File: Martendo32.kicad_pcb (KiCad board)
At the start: 2 copper layers, 75.2 x 98.5 mm, 104 parts, among them CN2 ZX-MX1.25-2PWT, J1 AudioJack4_SwitchTR1, J2 Conn_01x03, J4 USB-C, Q1 NPN, Q2 AO3401A, SW1 SK-3296S-01-L3, U3 TP4056, U4 NS4168, U5 TPS61040DBV, U6 AP2112K-3.3

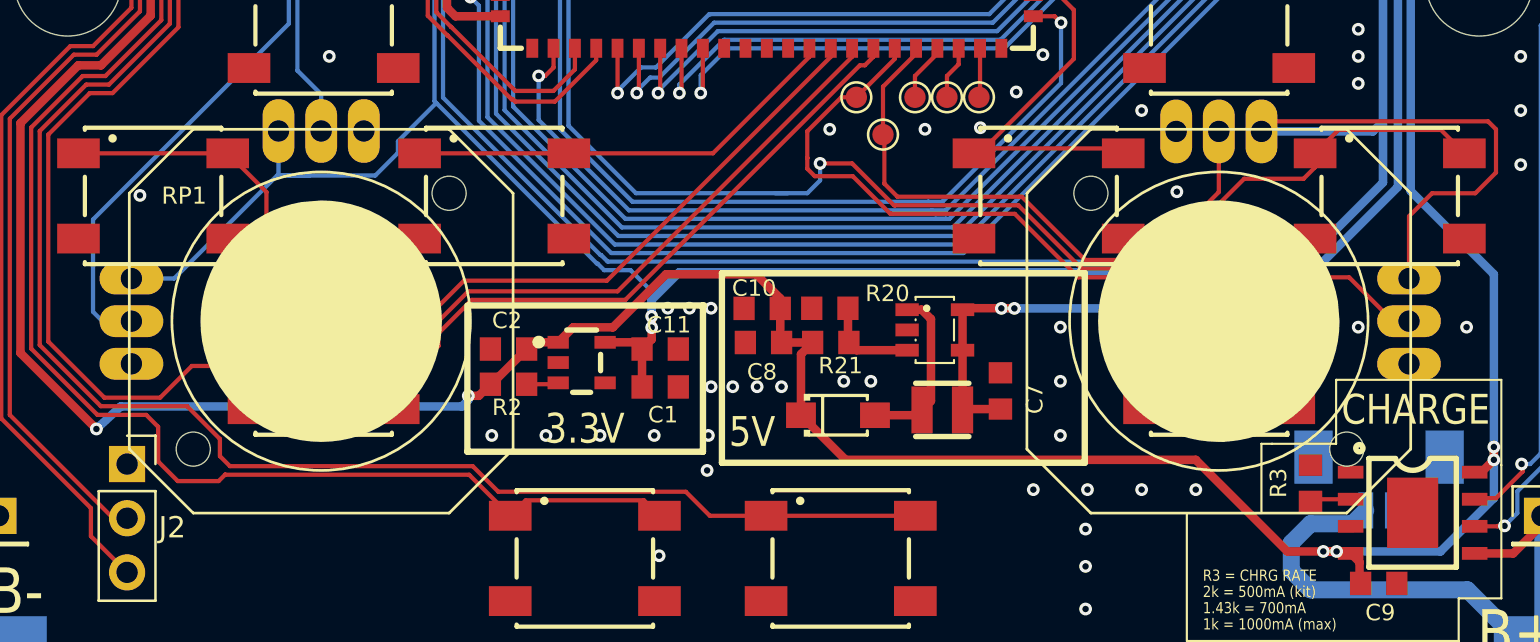
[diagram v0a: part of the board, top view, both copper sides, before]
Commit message: Add files via upload
improved Silkscreen
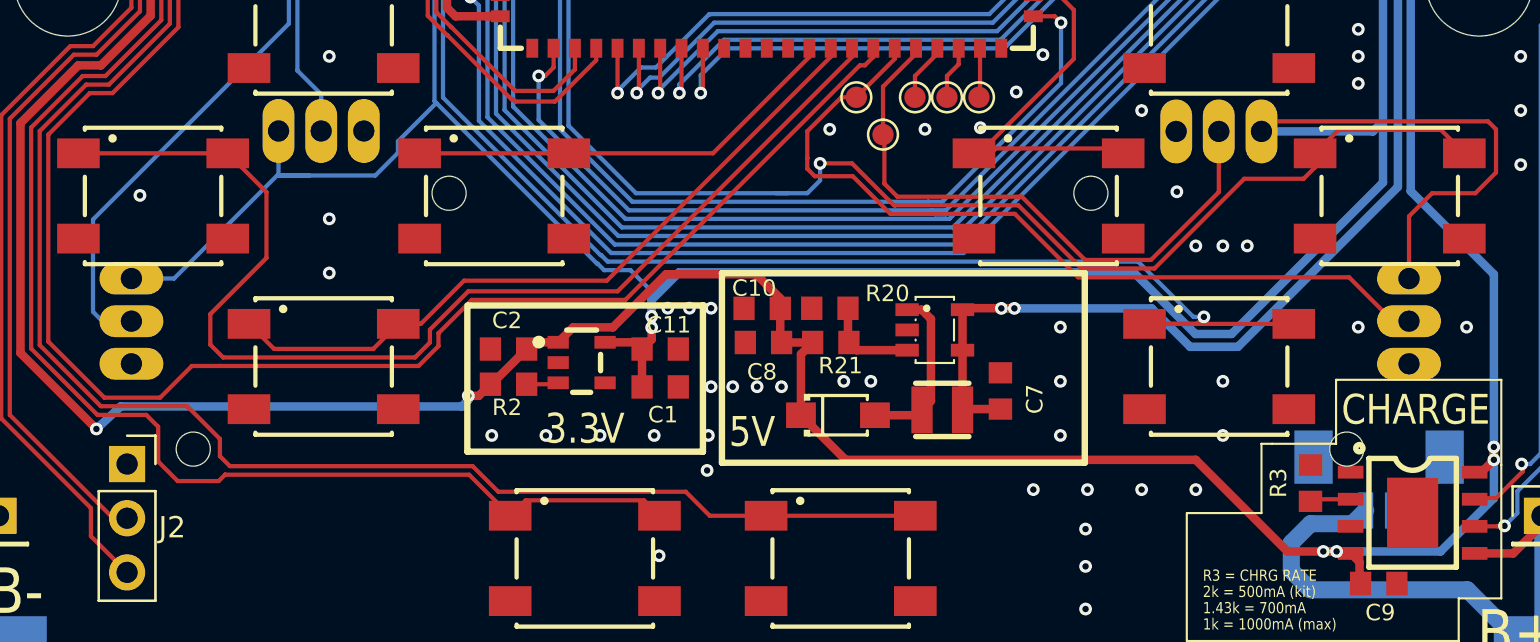
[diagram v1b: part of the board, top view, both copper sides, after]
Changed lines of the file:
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@@
 		(at 62.99 133.978 180)
 		(property "Reference" "RP1"
-			(at 6.428 5.882 0)
+			(at -0.126 5.882 0)
 			(unlocked yes)
 			(layer "F.SilkS")
+			(hide yes)
 			(effects
 				(font
@@
 		(sheetfile "Martendo32.kicad_sch")
 		(attr smd dnp)
-		(fp_line
-			(start 9 6)
-			(end 6 9)
-			(stroke
-				(width 0.127)
-				(type solid)
-			)
-			(layer "F.SilkS")
-		)
-		(fp_line
-			(start 9 -6)
-			(end 9 6)
-			(stroke
-				(width 0.127)
-				(type solid)
-			)
-			(layer "F.SilkS")
-		)
-		(fp_line
-			(start 6 9)
-			(end -6 9)
-			(stroke
-				(width 0.127)
-				(type solid)
-			)
-			(layer "F.SilkS")
-		)
-		(fp_line
-			(start 6 -9)
-			(end 9 -6)
-			(stroke
-				(width 0.127)
-				(type solid)
-			)
-			(layer "F.SilkS")
-		)
-		(fp_line
-			(start -6 9)
-			(end -9 6)
-			(stroke
-				(width 0.127)
-				(type solid)
-			)
-			(layer "F.SilkS")
-		)
-		(fp_line
-			(start -6 -9)
-			(end 6 -9)
-			(stroke
-				(width 0.127)
-				(type solid)
-			)
-			(layer "F.SilkS")
-		)
-		(fp_line
-			(start -9 6)
-			(end -9 -6)
-			(stroke
-				(width 0.127)
-				(type solid)
-			)
-			(layer "F.SilkS")
-		)
-		(fp_line
-			(start -9 -6)
-			(end -6 -9)
-			(stroke
-				(width 0.127)
-				(type solid)
-			)
-			(layer "F.SilkS")
-		)
-		(fp_circle
-			(center 0 0)
-			(end 0 7)
-			(stroke
-				(width 0.127)
-				(type solid)
-			)
-			(fill no)
-			(layer "F.SilkS")
-		)
-		(fp_poly
-			(pts
-				(xy 5.64421 0.467692) (xy 5.58631 0.932191) (xy 5.490251 1.390321) (xy 5.356688 1.838953) (xy 5.186532 2.275024)
-				(xy 4.980947 2.695554) (xy 4.741338 3.097671) (xy 4.46934 3.478627) (xy 4.166812 3.835821) (xy 3.835821 4.166812)
-				(xy 3.478627 4.46934) (xy 3.097671 4.741338) (xy 2.695554 4.980947) (xy 2.275024 5.186532) (xy 1.838953 5.356688)
-				(xy 1.390321 5.490251) (xy 0.930903 5.586581) (xy 0.001315 5.663609) (xy -0.467692 5.64421) (xy -0.932191 5.58631)
-				(xy -1.390321 5.490251) (xy -1.838953 5.356688) (xy -2.275024 5.186532) (xy -2.695554 4.980947)
-				(xy -3.097671 4.741338) (xy -3.478627 4.46934) (xy -3.835821 4.166812) (xy -4.166812 3.835821) (xy -4.46934 3.478627)
-				(xy -4.741338 3.097671) (xy -4.980947 2.695554) (xy -5.186532 2.275024) (xy -5.356688 1.838953)
-				(xy -5.490251 1.390321) (xy -5.58631 0.932191) (xy -5.64421 0.467692) (xy -5.663554 0) (xy -5.64421 -0.467692)
-				(xy -5.58631 -0.932191) (xy -5.490251 -1.390321) (xy -5.356688 -1.838953) (xy -5.186532 -2.275024)
-				(xy -4.980947 -2.695554) (xy -4.741338 -3.097671) (xy -4.46934 -3.478627) (xy -4.166812 -3.835821)
-				(xy -3.835821 -4.166812) (xy -3.478627 -4.46934) (xy -3.097671 -4.741338) (xy -2.695554 -4.980947)
-				(xy -2.275024 -5.186532) (xy -1.838953 -5.356688) (xy -1.390321 -5.490251) (xy -0.932191 -5.58631)
-				(xy -0.467692 -5.64421) (xy 0 -5.663554) (xy 0.467692 -5.64421) (xy 0.932191 -5.58631) (xy 1.390321 -5.490251)
-				(xy 1.838953 -5.356688) (xy 2.275024 -5.186532) (xy 2.695554 -4.980947) (xy 3.097671 -4.741338)
-				(xy 3.478627 -4.46934) (xy 3.835821 -4.166812) (xy 4.166812 -3.835821) (xy 4.46934 -3.478627) (xy 4.741338 -3.097671)
-				(xy 4.980947 -2.695554) (xy 5.186532 -2.275024) (xy 5.356688 -1.838953) (xy 5.490251 -1.390321)
-				(xy 5.58631 -0.932191) (xy 5.64421 -0.467692) (xy 5.663554 0)
-			)
-			(stroke
-				(width 0)
-				(type default)
-			)
-			(fill yes)
-			(layer "F.SilkS")
-		)
 		(pad "" np_thru_hole circle
 			(at -6 6 90)
@@
 		(at 105.09 133.978 90)
 		(property "Reference" "RP2"
-			(at 6.428 5.882 270)
+			(at 5.562 2.222 0)
 			(unlocked yes)
 			(layer "F.SilkS")
@@
 		(sheetfile "Martendo32.kicad_sch")
 		(attr smd dnp)
-		(fp_line
-			(start 6 -9)
-			(end 9 -6)
-			(stroke
-				(width 0.127)
-				(type solid)
-			)
-			(layer "F.SilkS")
-		)
-		(fp_line
-			(start -6 -9)
-			(end 6 -9)
-			(stroke
-				(width 0.127)
-				(type solid)
-			)
-			(layer "F.SilkS")
-		)
-		(fp_line
-			(start 9 -6)
-			(end 9 6)
-			(stroke
-				(width 0.127)
-				(type solid)
-			)
-			(layer "F.SilkS")
-		)
-		(fp_line
-			(start -9 -6)
-			(end -6 -9)
-			(stroke
-				(width 0.127)
-				(type solid)
-			)
-			(layer "F.SilkS")
-		)
-		(fp_line
-			(start 9 6)
-			(end 6 9)
-			(stroke
-				(width 0.127)
-				(type solid)
-			)
-			(layer "F.SilkS")
-		)
-		(fp_line
-			(start -9 6)
-			(end -9 -6)
-			(stroke
-				(width 0.127)
-				(type solid)
-			)
-			(layer "F.SilkS")
-		)
-		(fp_line
-			(start 6 9)
-			(end -6 9)
-			(stroke
-				(width 0.127)
-				(type solid)
-			)
-			(layer "F.SilkS")
-		)
-		(fp_line
-			(start -6 9)
-			(end -9 6)
-			(stroke
-				(width 0.127)
-				(type solid)
-			)
-			(layer "F.SilkS")
-		)
-		(fp_circle
-			(center 0 0)
-			(end 0 7)
-			(stroke
-				(width 0.127)
-				(type solid)
-			)
-			(fill no)
-			(layer "F.SilkS")
-		)
-		(fp_poly
-			(pts
-				(xy 5.64421 0.467692) (xy 5.58631 0.932191) (xy 5.490251 1.390321) (xy 5.356688 1.838953) (xy 5.186532 2.275024)
-				(xy 4.980947 2.695554) (xy 4.741338 3.097671) (xy 4.46934 3.478627) (xy 4.166812 3.835821) (xy 3.835821 4.166812)
-				(xy 3.478627 4.46934) (xy 3.097671 4.741338) (xy 2.695554 4.980947) (xy 2.275024 5.186532) (xy 1.838953 5.356688)
-				(xy 1.390321 5.490251) (xy 0.930903 5.586581) (xy 0.001315 5.663609) (xy -0.467692 5.64421) (xy -0.932191 5.58631)
-				(xy -1.390321 5.490251) (xy -1.838953 5.356688) (xy -2.275024 5.186532) (xy -2.695554 4.980947)
-				(xy -3.097671 4.741338) (xy -3.478627 4.46934) (xy -3.835821 4.166812) (xy -4.166812 3.835821) (xy -4.46934 3.478627)
-				(xy -4.741338 3.097671) (xy -4.980947 2.695554) (xy -5.186532 2.275024) (xy -5.356688 1.838953)
-				(xy -5.490251 1.390321) (xy -5.58631 0.932191) (xy -5.64421 0.467692) (xy -5.663554 0) (xy -5.64421 -0.467692)
-				(xy -5.58631 -0.932191) (xy -5.490251 -1.390321) (xy -5.356688 -1.838953) (xy -5.186532 -2.275024)
-				(xy -4.980947 -2.695554) (xy -4.741338 -3.097671) (xy -4.46934 -3.478627) (xy -4.166812 -3.835821)
-				(xy -3.835821 -4.166812) (xy -3.478627 -4.46934) (xy -3.097671 -4.741338) (xy -2.695554 -4.980947)
-				(xy -2.275024 -5.186532) (xy -1.838953 -5.356688) (xy -1.390321 -5.490251) (xy -0.932191 -5.58631)
-				(xy -0.467692 -5.64421) (xy 0 -5.663554) (xy 0.467692 -5.64421) (xy 0.932191 -5.58631) (xy 1.390321 -5.490251)
-				(xy 1.838953 -5.356688) (xy 2.275024 -5.186532) (xy 2.695554 -4.980947) (xy 3.097671 -4.741338)
-				(xy 3.478627 -4.46934) (xy 3.835821 -4.166812) (xy 4.166812 -3.835821) (xy 4.46934 -3.478627) (xy 4.741338 -3.097671)
-				(xy 4.980947 -2.695554) (xy 5.186532 -2.275024) (xy 5.356688 -1.838953) (xy 5.490251 -1.390321)
-				(xy 5.58631 -0.932191) (xy 5.64421 -0.467692) (xy 5.663554 0)
-			)
-			(stroke
-				(width 0)
-				(type default)
-			)
-			(fill yes)
-			(layer "F.SilkS")
-		)
 		(pad "" np_thru_hole circle
 			(at -6 6)
